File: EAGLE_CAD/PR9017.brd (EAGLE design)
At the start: 70 x 70 mm, 76 parts, among them SW1 C&K_PTS645, Y1 ABS25XTAL

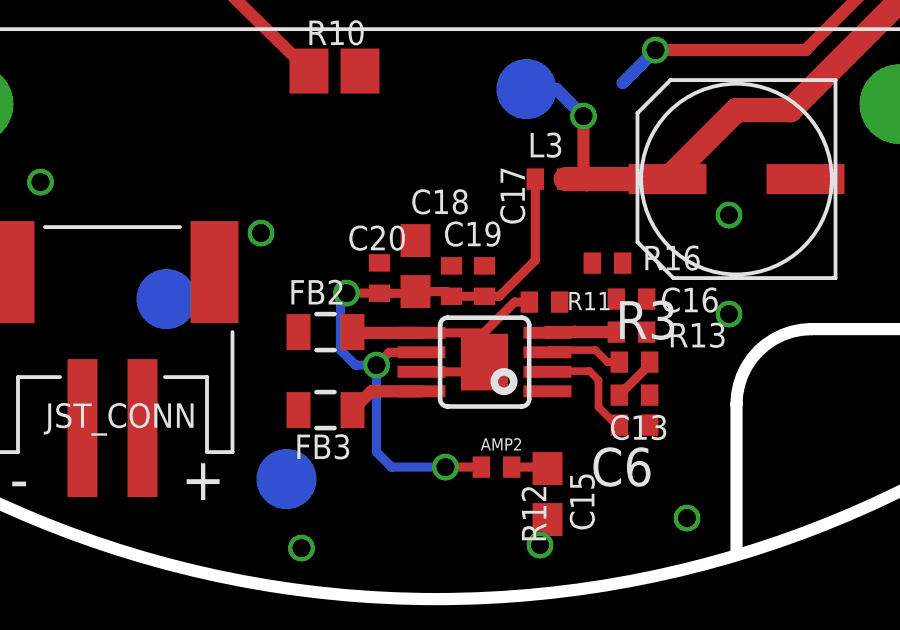
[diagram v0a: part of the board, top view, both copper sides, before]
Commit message: Updated Amp
Updated Amp SCH
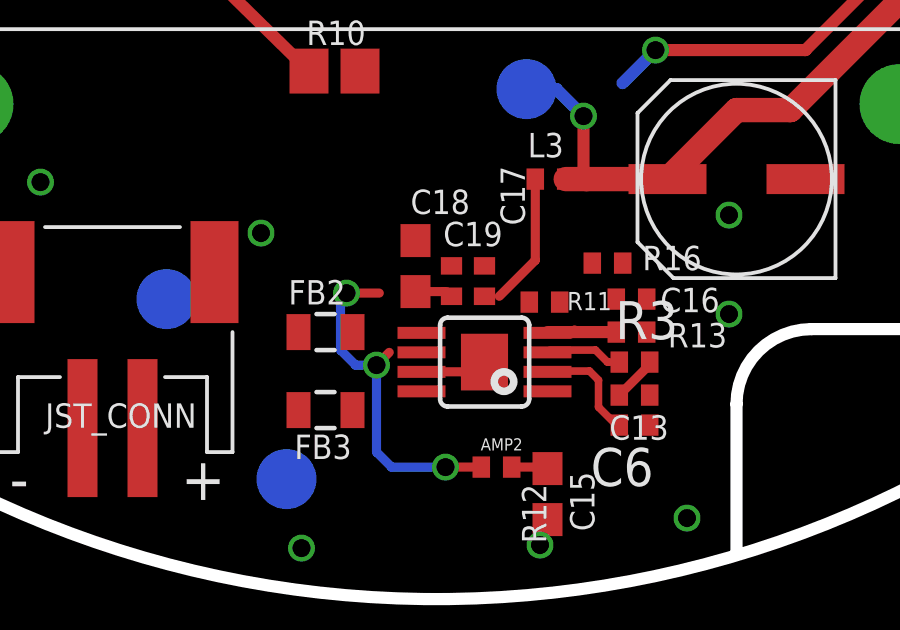
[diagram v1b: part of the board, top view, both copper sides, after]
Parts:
- removed C20: 100pf, PR_Parts_Library:C0402_WORTHINGTON
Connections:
- net GND: no longer C20.2
- net N$14: now also AMP2.4; no longer AMP2.3
- net N$2: no longer C20.1
- net N$5: now also AMP2.3; no longer AMP2.4
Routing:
- net N$4: track 6.33 -> 0.00 mm
- net N$2: track 21.3 -> 17.2 mm
- net N$11: track 2.56 -> 0.00 mm
